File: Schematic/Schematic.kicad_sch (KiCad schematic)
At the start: 2 parts

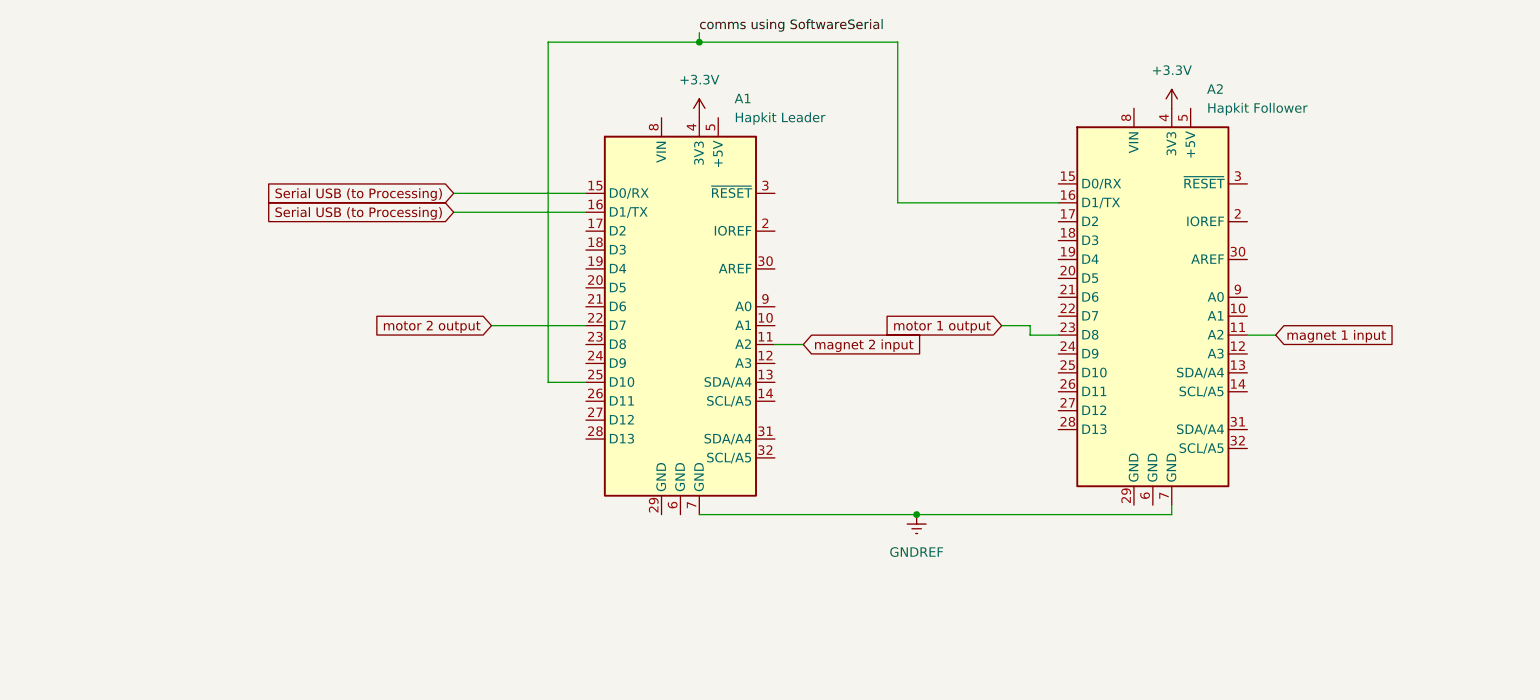
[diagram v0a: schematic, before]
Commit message: updated schematic
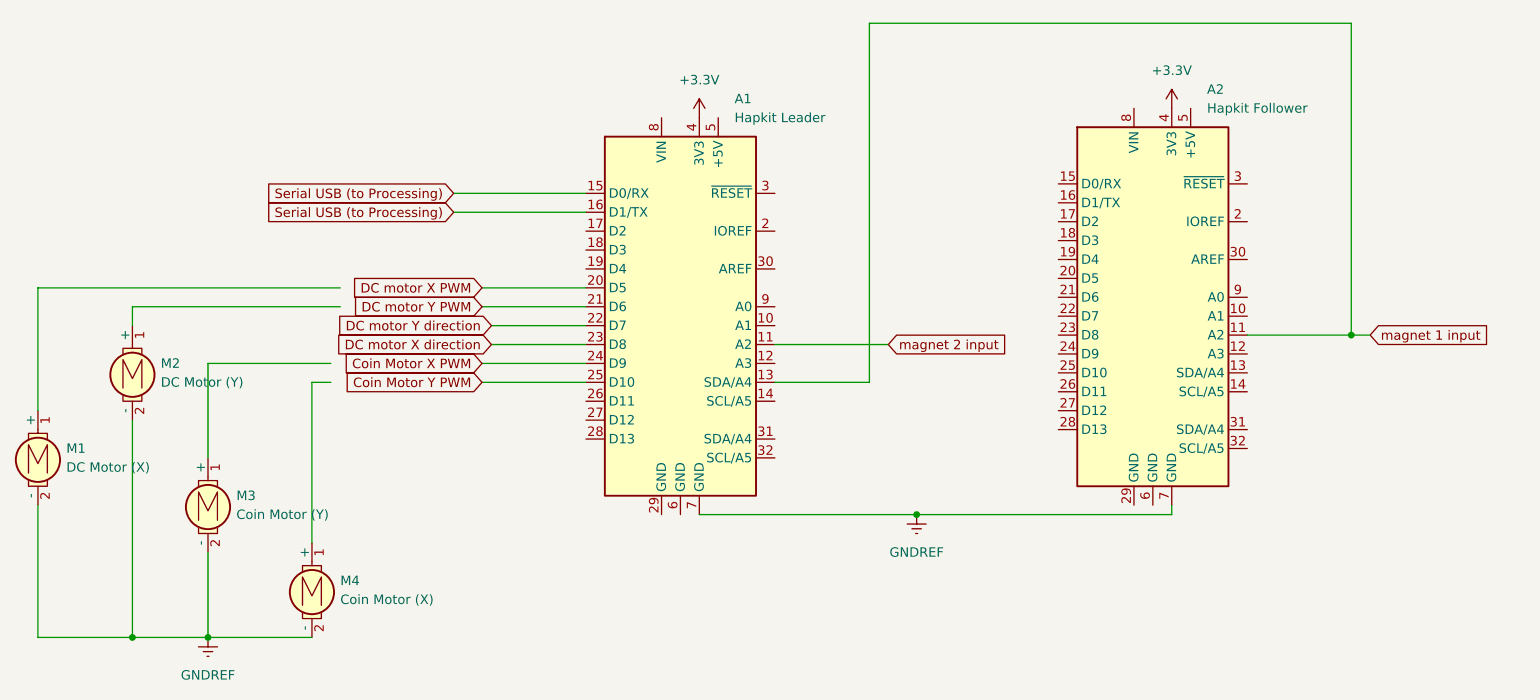
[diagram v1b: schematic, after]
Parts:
- added M1: DC Motor (X), symbol ME218_BaseLib:Motor
- added M2: DC Motor (Y), symbol ME218_BaseLib:Motor
- added M3: Coin Motor (Y), symbol ME218_BaseLib:Motor
- added M4: Coin Motor (X), symbol ME218_BaseLib:Motor
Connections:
- net GNDREF: now also M1.2 (-), M2.2 (-), M3.2 (-), M4.2 (-)
- net magnet 1 input: now also A1.13 (SDA/A4)
- net DC motor X PWM: now reaches A1.20 (D5)
- net DC motor Y PWM: now reaches A1.21 (D6)
- net DC motor X direction: now reaches A1.23 (D8)
- net Coin Motor X PWM: now reaches A1.24 (D9)
- net comms using SoftwareSerial: no longer names the net of A2.16 (D1/TX)
- net comms using SoftwareSerial: no longer A1.25 (D10)
- net motor 1 output: no longer names the net of A2.23 (D8)
- net motor 2 output renamed DC motor Y direction
- new net Coin Motor Y PWM: A1.25 (D10)
